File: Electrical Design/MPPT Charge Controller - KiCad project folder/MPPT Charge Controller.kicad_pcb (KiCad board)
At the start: 4 copper layers, 35.6 x 60 mm, 53 parts, among them Q1 SI7272DP, Q3 2N7002, U2 AP63203WU, U3 ACS712-20A, U4 ACS712-20A, U5 MCP4018

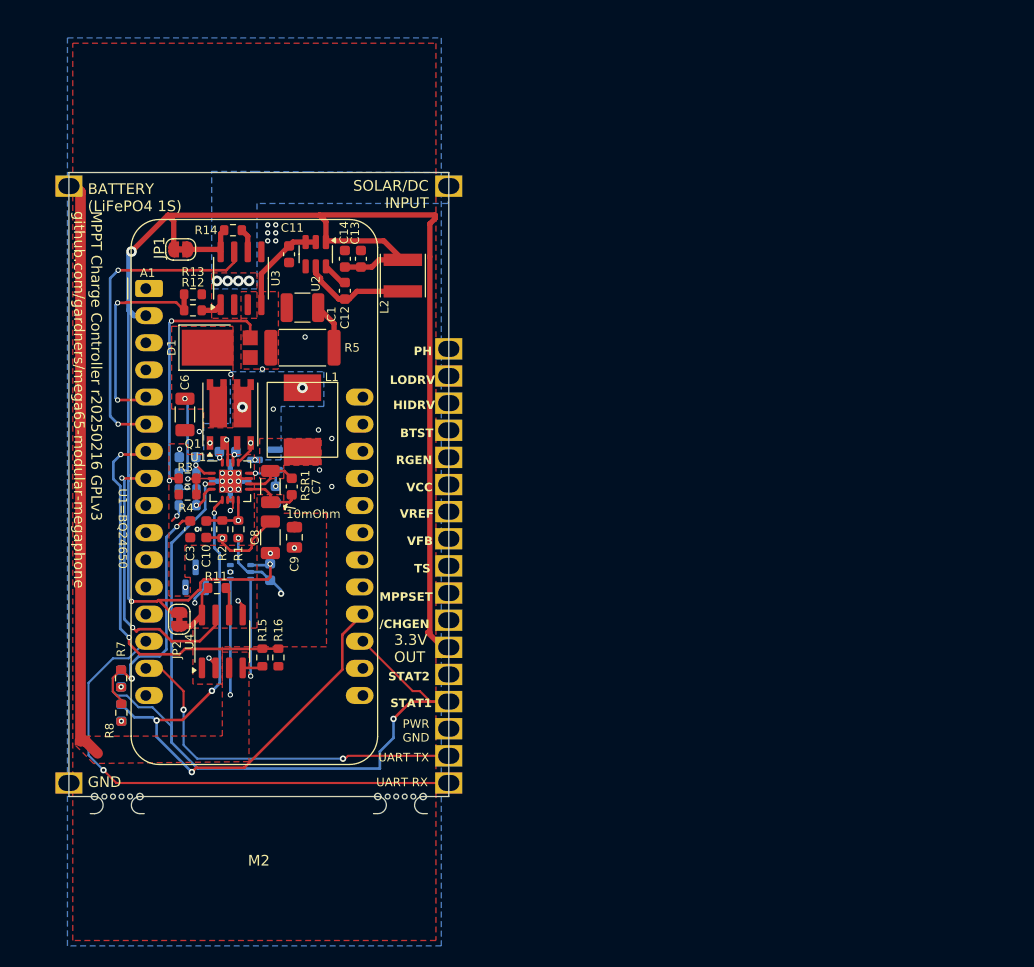
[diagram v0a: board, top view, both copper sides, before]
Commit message: finish panelising
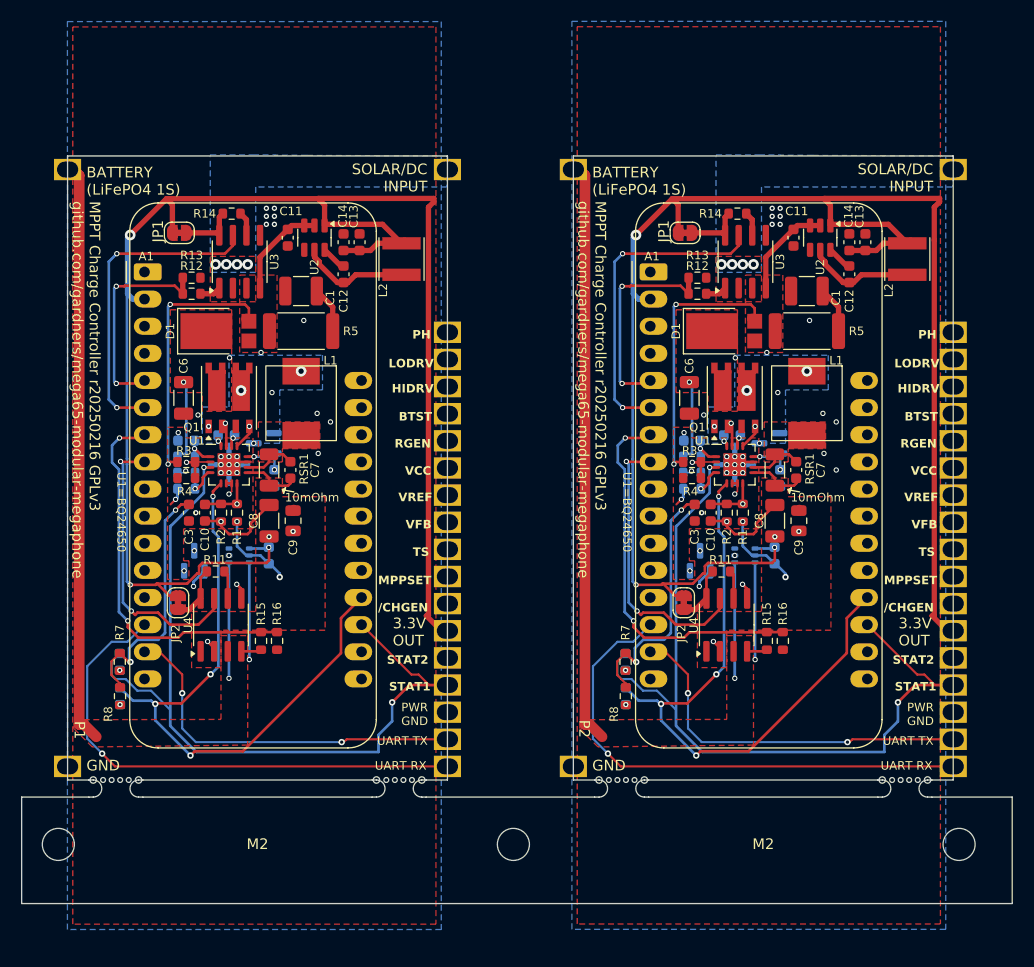
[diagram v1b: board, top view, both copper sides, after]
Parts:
- added A1: Adafruit_Feather_HUZZAH32_ESP32, Module:Adafruit_Feather, F.Cu at (157.2, 98.5)
- added C1: 2.2uF, Capacitor_SMD:C_1210_3225Metric, F.Cu at (161.7, 81.2)
- added C10: 22pF, Capacitor_SMD:C_0603_1608Metric, F.Cu at (152.7, 102.0)
- added C11: 10uF, Capacitor_SMD:C_0603_1608Metric, F.Cu at (160.5, 76.2)
- added C12: 0.1uF, Capacitor_SMD:C_0603_1608Metric, F.Cu at (165.7, 79.6)
- added C13: 22uF, Capacitor_SMD:C_0603_1608Metric, F.Cu at (167.2, 76.6)
- added C14: 22uF, Capacitor_SMD:C_0603_1608Metric, F.Cu at (165.7, 76.6)
- added C15: 0.1uF, Capacitor_SMD:C_0603_1608Metric, B.Cu at (158.7, 106.0)
- added C2: C2=1uF, Capacitor_SMD:C_0603_1608Metric, B.Cu at (151.0, 95.2)
- added C3: 1uF, Capacitor_SMD:C_0603_1608Metric, F.Cu at (151.2, 102.0)
- added C4: 1uF, Capacitor_SMD:C_0603_1608Metric, B.Cu at (159.2, 98.7)
- added C5: 0.1uF, Capacitor_SMD:C_0603_1608Metric, B.Cu at (154.7, 94.7)
- added C6: 10uF, Capacitor_SMD:C_1206_3216Metric, F.Cu at (150.7, 91.2)
- added C7: 0.1uF, Capacitor_SMD:C_0603_1608Metric, F.Cu at (160.7, 98.0)
- added C8: 10uF, Capacitor_SMD:C_1206_3216Metric, F.Cu at (158.7, 102.7)
- added C9: 4.7uF, Capacitor_SMD:C_0805_2012Metric, F.Cu at (161.0, 102.7)
- added D1: PDS1040, Diode_SMD:D_PowerDI-5, F.Cu at (154.0, 85.0)
- added D2: BAT54C, Package_TO_SOT_SMD:SOT-23, B.Cu at (158.2, 95.5)
- added D3: RED, LED_SMD:LED_0603_1608Metric, B.Cu at (144.8, 115.9)
- added D4: GREEN, LED_SMD:LED_0603_1608Metric, B.Cu at (144.8, 119.1)
- added JP1: Jumper_2_Bridged, Jumper:SolderJumper-2_P1.3mm_Bridged_RoundedPad1.0x1.5mm, F.Cu at (150.3, 75.8)
- added JP2: Jumper_2_Bridged, Jumper:SolderJumper-2_P1.3mm_Bridged_RoundedPad1.0x1.5mm, F.Cu at (150.2, 110.4)
- added L1: 10uH, MPPT Charge Controller Footprint Library:L_Vishay_6.9x6.5, F.Cu at (161.7, 91.7)
- added L2: 4.7uH, Inductor_SMD:L_Vishay_IFSC-1515AH_4x4x1.8mm, F.Cu at (171.1, 78.2)
- added M2: ~, MegaCastle:MegaCastle2x23-Module-I30.0x53.6-M80000307FFFC-PANEL, F.Cu at (157.6, 97.8)
- added NT1: ~, NetTie:NetTie-2_SMD_Pad0.5mm, B.Cu at (156.2, 97.5)
- added NT2: ~, NetTie:NetTie-2_SMD_Pad0.5mm, B.Cu at (155.0, 96.2)
- added NT3: ~, NetTie:NetTie-2_SMD_Pad0.5mm, B.Cu at (153.7, 97.5)
- added NT4: ~, NetTie:NetTie-2_SMD_Pad0.5mm, B.Cu at (155.0, 98.7)
- added Q1: SI7272DP, Package_SO:PowerPAK_SO-8_Dual, F.Cu at (155.0, 91.2)
- added Q3: 2N7002, Package_TO_SOT_SMD:SOT-23, B.Cu at (151.7, 106.5)
- added R1: 100k, Resistor_SMD:R_0603_1608Metric, F.Cu at (155.7, 102.0)
- added R10: R10=30.1k, Resistor_SMD:R_0603_1608Metric, B.Cu at (151.0, 99.7)
- added R11: 100k, Resistor_SMD:R_0603_1608Metric, F.Cu at (153.7, 107.5)
- added R12: 499k, Resistor_SMD:R_0603_1608Metric, F.Cu at (151.5, 81.5)
- added R13: 36k, Resistor_SMD:R_0603_1608Metric, F.Cu at (151.5, 80.0)
- added R14: 100k, Resistor_SMD:R_0603_1608Metric, F.Cu at (155.2, 74.0)
- added R15: 499k, Resistor_SMD:R_0603_1608Metric, F.Cu at (158.0, 114.0)
- added R16: 100k, Resistor_SMD:R_0603_1608Metric, F.Cu at (159.5, 114.0)
- added R2: 140K, Resistor_SMD:R_0603_1608Metric, F.Cu at (154.2, 102.0)
- added R3: 499k, Resistor_SMD:R_0603_1608Metric, F.Cu at (151.0, 97.2)
- added R4: DNP, Resistor_SMD:R_0603_1608Metric, F.Cu at (151.0, 98.7)
- added R5: 2 Ohm, Resistor_SMD:R_2512_6332Metric, F.Cu at (161.7, 85.0)
- added R6: R6=10, Resistor_SMD:R_0603_1608Metric, B.Cu at (151.0, 96.7)
- added R7: 100, Resistor_SMD:R_0603_1608Metric, F.Cu at (144.8, 115.9)
- added R8: 100, Resistor_SMD:R_0603_1608Metric, F.Cu at (144.8, 119.1)
- added R9: R9=5.23k, Resistor_SMD:R_0603_1608Metric, B.Cu at (151.0, 98.2)
- added RSR1: 10mOhm, Resistor_SMD:R_1206_3216Metric, F.Cu at (158.7, 98.0)
- added U1: ~, MPPT Charge Controller Footprint Library:VQFN-16_EP_3.5x3.5_Pitch0.5mm, F.Cu at (155.0, 97.5)
- added U2: AP63203WU, Package_TO_SOT_SMD:TSOT-23-6, F.Cu at (163.0, 76.2)
- added U3: ACS712-20A, Package_SO:SOIC-8_3.9x4.9mm_P1.27mm, F.Cu at (156.0, 78.5)
- added U4: ACS712-20A, Package_SO:SOIC-8_3.9x4.9mm_P1.27mm, F.Cu at (154.2, 112.5)
- added U5: MCP4018, Package_TO_SOT_SMD:SOT-363_SC-70-6, B.Cu at (155.9, 106.0)
- moved D3 1.56 mm to (97.4, 115.9)
- moved R7 1.56 mm to (97.4, 115.9)
- moved A1 1.56 mm to (109.9, 98.5)
- moved C1 1.56 mm to (114.4, 81.2)
- moved C10 1.56 mm to (105.4, 102.0)
- moved C11 1.56 mm to (113.1, 76.2)
- moved C12 1.56 mm to (118.3, 79.6)
- moved C13 1.56 mm to (119.8, 76.6)
- moved C14 1.56 mm to (118.3, 76.6)
- moved C15 1.56 mm to (111.3, 106.0)
- moved C2 1.56 mm to (103.6, 95.2)
- moved C3 1.56 mm to (103.9, 102.0)
- moved C4 1.56 mm to (111.9, 98.7)
- moved C5 1.56 mm to (107.4, 94.7)
- moved C6 1.56 mm to (103.4, 91.2)
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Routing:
- net +3.3V: track 147.2 -> 294.5 mm, vias 3 -> 6
- net /STAT1: track 79.1 -> 158.2 mm, vias 2 -> 4
- net /STAT2: track 69.8 -> 139.5 mm, vias 4 -> 8
- net VBAT_OUT: track 56.7 -> 113.4 mm
- net UART_RX: track 48.6 -> 97.1 mm, vias 1 -> 2
- net /VREF: track 48.5 -> 97.1 mm, vias 4 -> 8
- net /MPPSET: track 37.4 -> 74.8 mm, vias 3 -> 6
- net /Battery Voltage: track 35.7 -> 71.4 mm, vias 2 -> 4
- net UART_TX: track 34.9 -> 69.9 mm, vias 2 -> 4
- net /VCC: track 34.8 -> 69.5 mm, vias 4 -> 8
- net /VIN: track 34.3 -> 68.5 mm, vias 2 -> 4
- net PWR_GND: track 32.7 -> 65.4 mm, vias 14 -> 28
- net /TS: track 31.1 -> 62.2 mm, vias 2 -> 4
- net /HIDRV: track 30.0 -> 59.9 mm, vias 2 -> 4
- net /Solar Current: track 29.8 -> 59.5 mm, vias 2 -> 4
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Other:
- outline, holes or cut-outs redrawn
- board text added: "P1"
- board text added: "P2"
